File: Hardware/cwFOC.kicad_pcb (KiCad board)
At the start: 2 copper layers, 46 x 46 mm, 53 parts, among them J1 Motor, J2 Debug, J3 KF2EDGV, U1 MP6540, U2 AS5600, U3 HT7533, U4 HT7150, U5 MAX3485, U6 CW32F030K8

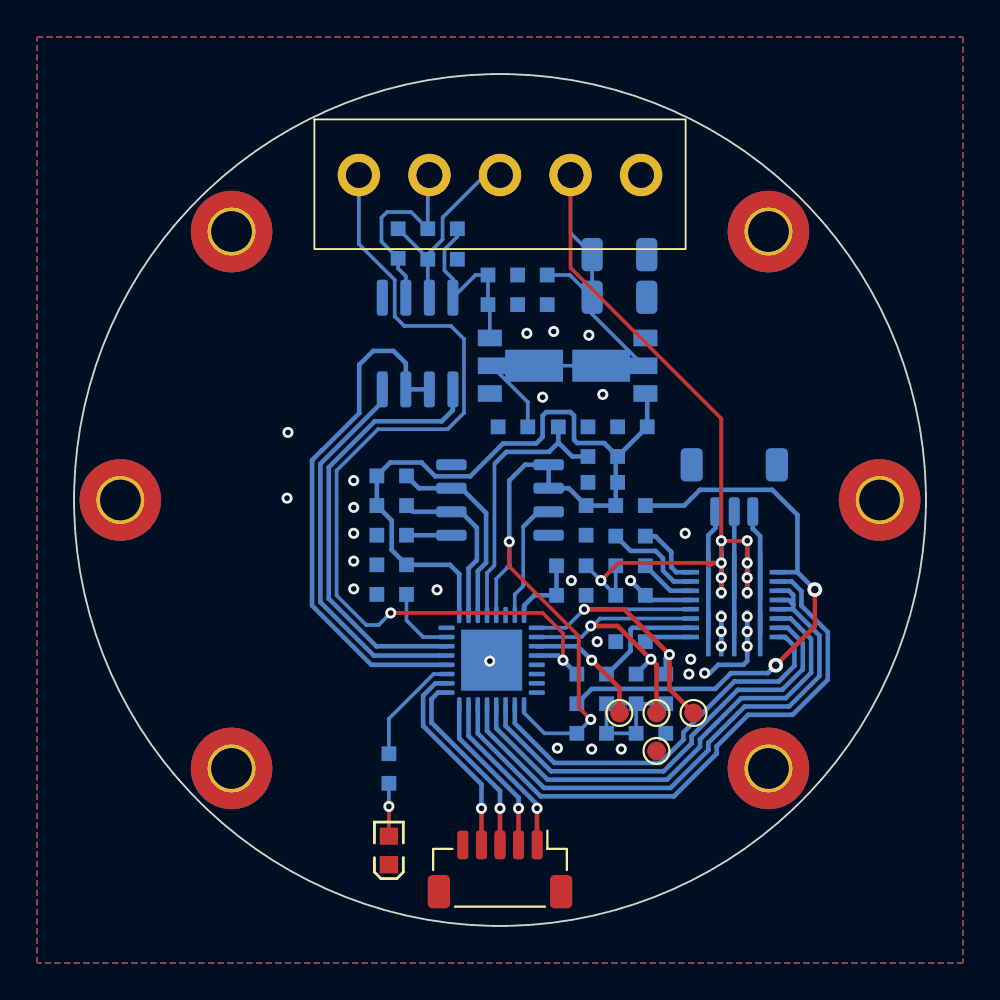
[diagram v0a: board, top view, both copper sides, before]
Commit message: 基本完成PCB设计
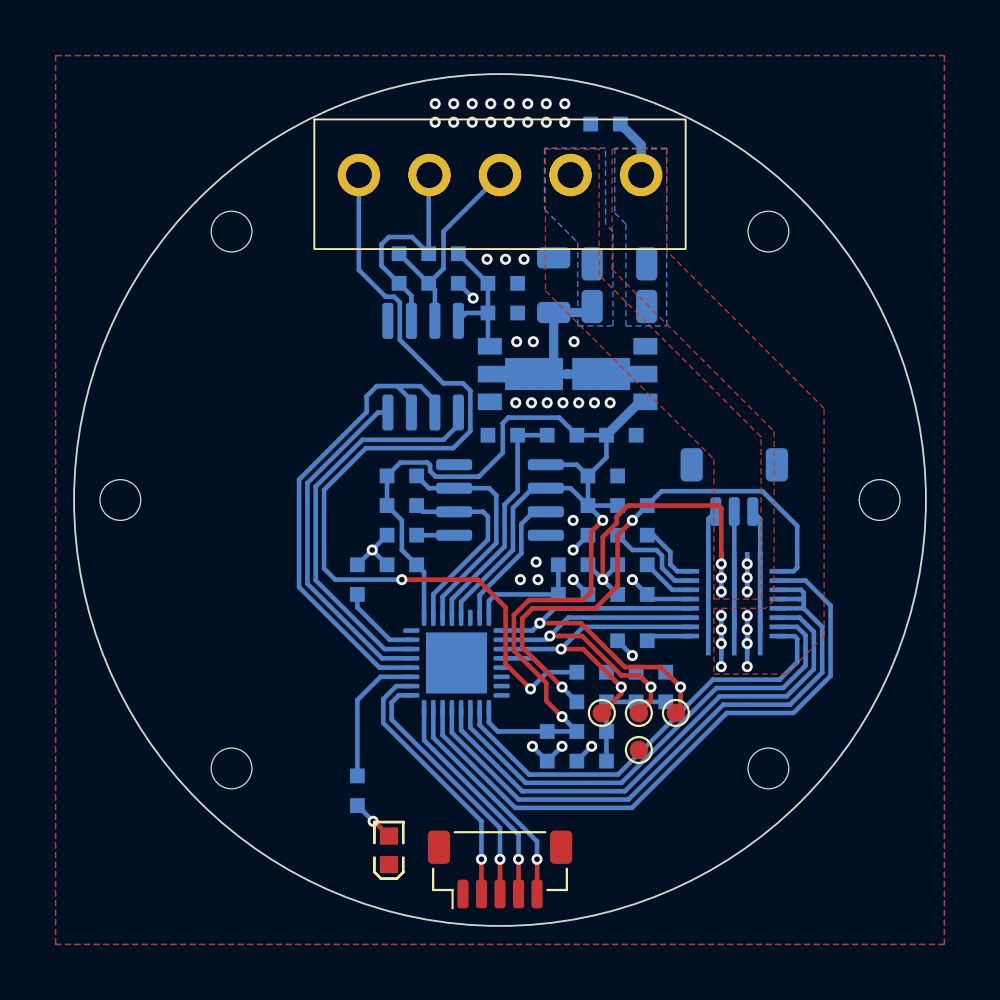
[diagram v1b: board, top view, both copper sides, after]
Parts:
- removed C15: 4.7uF, myDevice:0603_C
- added C4: 10uF, Capacitor_SMD:C_1206_3216Metric, B.Cu at (142.9, 78.4)
- added R19: 0R, myDevice:0603_R, B.Cu at (145.7, 69.7)
- C3: value 4.7uF -> 100nF
- H1, H2, H3, H4, H5, H6: footprint MountingHole:MountingHole_2.2mm_M2_Pad_TopBottom -> myLib:MountingHole_2.2mm_M2
- R15: value 10K -> 22R
- U2: footprint Package_SO:SOP-8_3.9x4.9mm_P1.27mm -> Package_SO:SOIC-8_3.9x4.9mm_P1.27mm
- moved C3 17.3 mm to (142.6, 103.3), turned to -90 degrees
- moved C2 3.83 mm to (140.2, 86.5), turned to 0 degrees
- moved R9 3.53 mm to (144.9, 104.1), turned to 180 degrees
- moved R10 2.48 mm to (143.3, 86.5)
- moved R16 2.08 mm to (132.3, 105.7)
- moved R7 2.02 mm to (132.3, 94.3), turned to -90 degrees
- moved U6 1.91 mm to (137.7, 98.8)
- moved R14 1.35 mm to (136.9, 76.7)
- moved R12 1.35 mm to (134.6, 77.5)
- moved R11 1.30 mm to (136.9, 78.3)
- moved U5 1.29 mm to (135.8, 82.8)
- moved TP4 0.95 mm to (147.5, 103.5)
- moved TP1 0.95 mm to (149.5, 101.5)
- moved TP2 0.95 mm to (147.5, 101.5)
- moved TP3 0.95 mm to (145.5, 101.5)
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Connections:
- net /MCU/UART2_RXD renamed /MCU/UART3_RXD
- net /MCU/UART2_TXD renamed /MCU/UART3_TXD
- C3 pad 1: VBUS -> +3V3
- C8 pad 2: GND -> GNDPWR
- C9 pad 2: GND -> GNDPWR
- J2 pad 1: /MCU/SWDIO -> GND
- J2 pad 2: /MCU/SWCLK -> /MCU/TXD
- J2 pad 4: /MCU/TXD -> /MCU/SWCLK
- J2 pad 5: GND -> /MCU/SWDIO
- J3 pad 5: GND -> GNDPWR
- U1 pad 10: GND -> GNDPWR
- U1 pad 12: GND -> GNDPWR
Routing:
- net VBUS: track 72.4 -> 33.2 mm, vias 9 -> 7
- net GND: track 7.95 -> 14.9 mm, vias 30 -> 42
- net GNDPWR: track 0.00 -> 6.91 mm, vias 0 -> 8
- net +3V3: track 66.5 -> 70.3 mm
- net /Driver/SOA: track 14.1 -> 17.8 mm, vias 1 -> 2
- net /Driver/ENA: track 31.0 -> 34.7 mm
- net /MCU/RXD: track 10.4 -> 14.0 mm
- net /MCU/TXD: track 10.9 -> 14.5 mm
- net /MCU/SWCLK: track 8.86 -> 12.1 mm
- net /MCU/SWDIO: track 9.07 -> 12.4 mm
- net /Driver/SOC: track 19.2 -> 22.4 mm
- net /Driver/SOB: track 16.9 -> 20.1 mm
- net BRK: track 49.2 -> 51.9 mm
- net /Driver/nSLP: track 31.5 -> 34.2 mm
- net +5V: track 10.0 -> 7.48 mm
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- added copper zone on B.Cu, net GNDPWR
- added copper zone on F.Cu, net GNDPWR
- added copper zone on B.Cu, net VBUS
- added copper zone on F.Cu, net VBUS
